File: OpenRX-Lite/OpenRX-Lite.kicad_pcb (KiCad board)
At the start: 6 copper layers, 8.2 x 12.2 mm, 39 parts, among them U1 ESP32-C3FH4, U2 TLV75533PDQNR, U3 SX1281IMLTRT, X1 CJ17-400001010B20

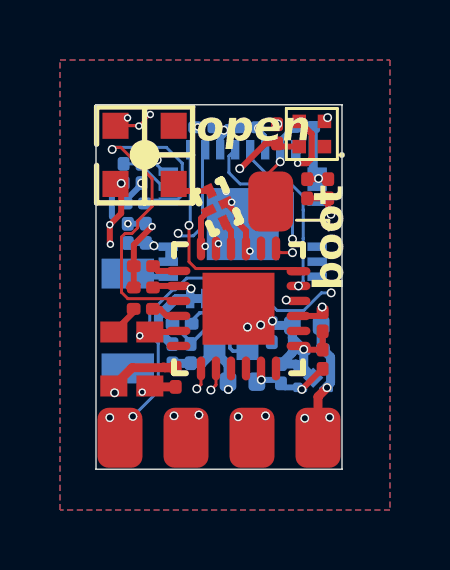
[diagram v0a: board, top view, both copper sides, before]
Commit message: final route
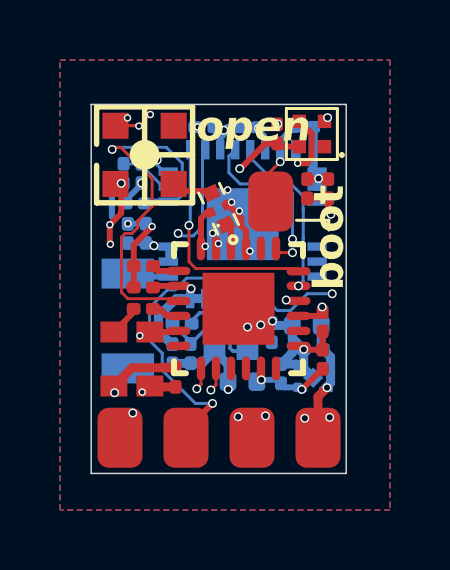
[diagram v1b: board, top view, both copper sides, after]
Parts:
- FL1: value 2450FM07D0034 -> 2450FM07D0034T; footprint OpenRX-Shared:FILTER-SMD_4P-L1.0-W0.5-L_DEA102700LT-XXX -> OpenRX-Shared:FILTER-SMD_4P-L1.0-W0.5-L
- moved TP1 2.20 mm to (180.0, 101.7)
- moved TP2 2.20 mm to (182.2, 101.7)
- moved FL1 0.08 mm to (183.3, 94.0)
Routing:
- net Net-(U1-U0RXD): track 10.7 -> 11.9 mm, vias 3 -> 2
- net Net-(U1-U0TXD): track 9.84 -> 10.1 mm, vias 2 -> 1
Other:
- board size 8.2 x 12.2 mm -> 8.5 x 12.3 mm
